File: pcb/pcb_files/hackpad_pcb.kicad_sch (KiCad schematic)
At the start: 1 part, among them U1 MOUDLE-SEEEDUINO-XIAO

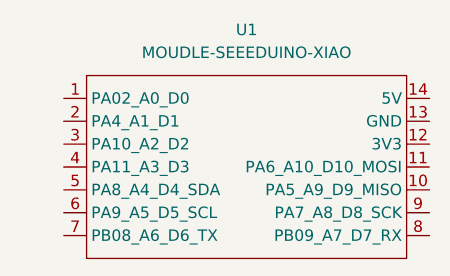
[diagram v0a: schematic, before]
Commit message: a
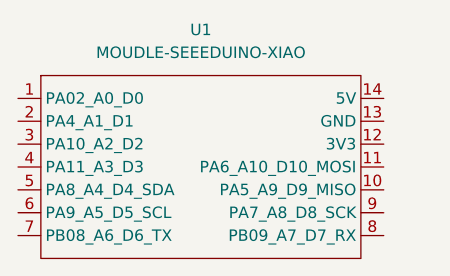
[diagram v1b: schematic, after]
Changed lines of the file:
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@@
 	(symbol
 		(lib_id "XIAO_RP2040:MOUDLE-SEEEDUINO-XIAO")
-		(at 115.57 96.52 0)
+		(at 110.49 96.52 0)
 		(unit 1)
 		(body_style 1)
@@
 		(fields_autoplaced yes)
 		(property "Reference" "U1"
-			(at 116.84 81.28 0)
+			(at 111.76 81.28 0)
 			(show_name no)
 			(do_not_autoplace no)
@@
 		)
 		(property "Value" "MOUDLE-SEEEDUINO-XIAO"
-			(at 116.84 83.82 0)
+			(at 111.76 83.82 0)
 			(show_name no)
 			(do_not_autoplace no)
@@
 		)
 		(property "Footprint" ""
-			(at 99.06 93.98 0)
+			(at 93.98 93.98 0)
 			(hide yes)
 			(show_name no)
@@
 		)
 		(property "Datasheet" ""
-			(at 99.06 93.98 0)
+			(at 93.98 93.98 0)
 			(hide yes)
 			(show_name no)
@@
 		)
 		(property "Description" ""
-			(at 115.57 96.52 0)
+			(at 110.49 96.52 0)
 			(hide yes)
 			(show_name no)
@@
 			)
 		)
+		(pin "9"
+		)
+		(pin "3"
+		)
+		(pin "5"
+		)
+		(pin "7"
+		)
 		(pin "1"
 		)
-		(pin "6"
+		(pin "14"
 		)
 		(pin "10"
@@
 		(pin "11"
 		)
-		(pin "3"
+		(pin "6"
+		)
+		(pin "13"
 		)
 		(pin "8"
@@
 		(pin "2"
 		)
-		(pin "5"
-		)
-		(pin "7"
-		)
-		(pin "9"
-		)
 		(pin "12"
 		)
-		(pin "14"
-		)
-		(pin "13"
-		)
 		(instances
